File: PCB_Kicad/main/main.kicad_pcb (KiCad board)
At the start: 2 copper layers, 59.9 x 31.5 mm, 28 parts, among them Q1 Q_NMOS_GDS, Q2 Q_NMOS_GDS, U1 LTC3854EMSEPBF, U2 ACS70331EESATR-005U3

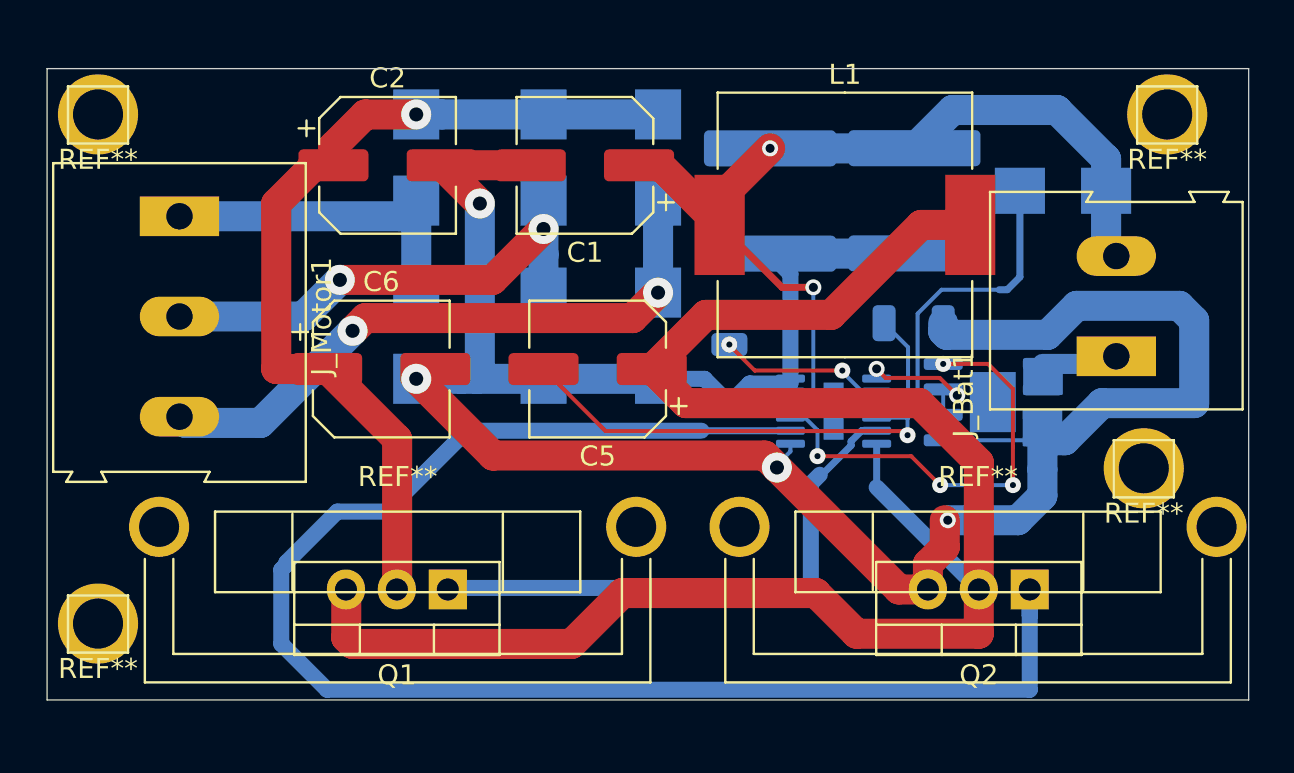
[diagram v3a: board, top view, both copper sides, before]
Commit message: kicad_updated
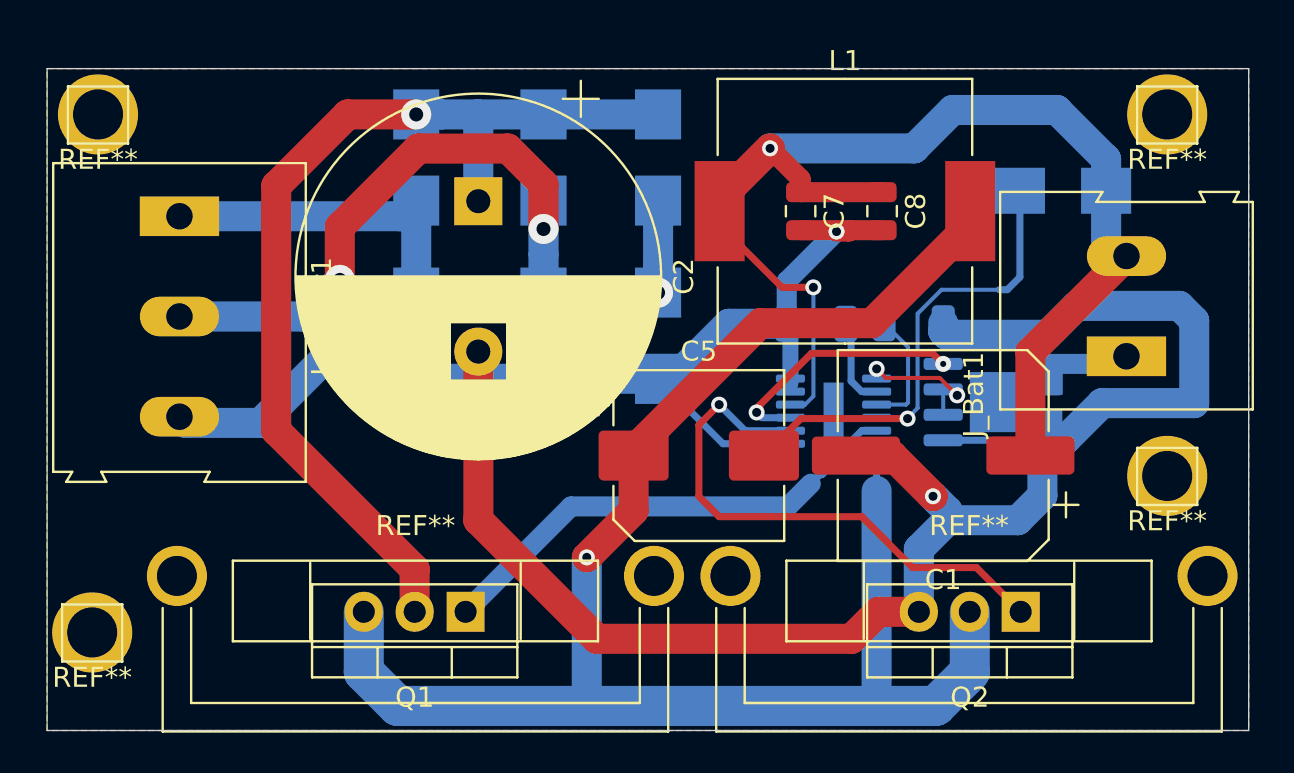
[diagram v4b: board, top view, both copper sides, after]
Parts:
- removed C6: 68uF, Capacitor_SMD:CP_Elec_6.3x7.7
- C1: footprint Capacitor_SMD:CP_Elec_6.3x7.7 -> Capacitor_SMD:CP_Elec_10x7.9
- C2: footprint Capacitor_SMD:CP_Elec_6.3x7.7 -> Capacitor_THT:CP_Radial_D18.0mm_P7.50mm
- C5: footprint Capacitor_SMD:CP_Elec_6.3x7.7 -> Capacitor_SMD:CP_Elec_8x10
- C7, C8: footprint Capacitor_SMD:C_2225_5664Metric_Pad1.80x6.60mm_HandSolder -> Capacitor_SMD:C_0805_2012Metric; moved to F.Cu
- moved C1 23.0 mm to (57.4, 38.6)
- moved C5 6.64 mm to (45.2, 38.6), turned to 0 degrees
- moved C3 5.01 mm to (51.1, 32.0), turned to 180 degrees
- moved C2 4.87 mm to (34.2, 25.9), turned to 270 degrees
- moved REF** 2.60 mm to (19.2, 44.6)
- moved REF** 2.49 mm to (46.8, 44.6)
- moved C8 1.69 mm to (54.4, 26.4)
- moved C7 1.61 mm to (50.3, 26.4)
- moved Q1 1.43 mm to (33.6, 46.4)
- moved REF** 1.23 mm to (68.6, 39.6)
- moved Q2 1.20 mm to (61.3, 46.4)
- moved L1 0.69 mm to (52.5, 26.4)
- moved REF** 0.53 mm to (15.0, 47.4)
- moved J_Bat1 0.51 mm to (66.5, 33.7)
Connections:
- REF** pad 1: (no net) -> GND (x4)
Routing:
- net Net-(Q2-Pad1): track 76.8 -> 27.5 mm, vias 0 -> 1
- net V_Bat: track 46.4 -> 60.0 mm
- net Net-(C5-Pad2): track 37.7 -> 25.3 mm
- net Net-(U1-Pad9): track 22.6 -> 13.9 mm, vias 4 -> 2
- net Net-(D_B1-Pad2): track 24.6 -> 30.7 mm
- net Net-(C2-Pad1): track 44.6 -> 49.0 mm
- net SW: track 91.1 -> 86.9 mm, vias 0 -> 1
- net TG: track 27.8 -> 24.4 mm
- net Net-(C3-Pad1): track 8.48 -> 5.18 mm, vias 2 -> 0
- net GND: track 130.8 -> 129.0 mm, vias 4 -> 2
- added copper zone on B.Cu, net GND
- added copper zone on F.Cu, net GND
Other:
- board size 59.9 x 31.5 mm -> 59.9 x 33 mm
